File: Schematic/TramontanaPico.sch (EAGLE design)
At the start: 15 parts, among them U4 TEMT6000

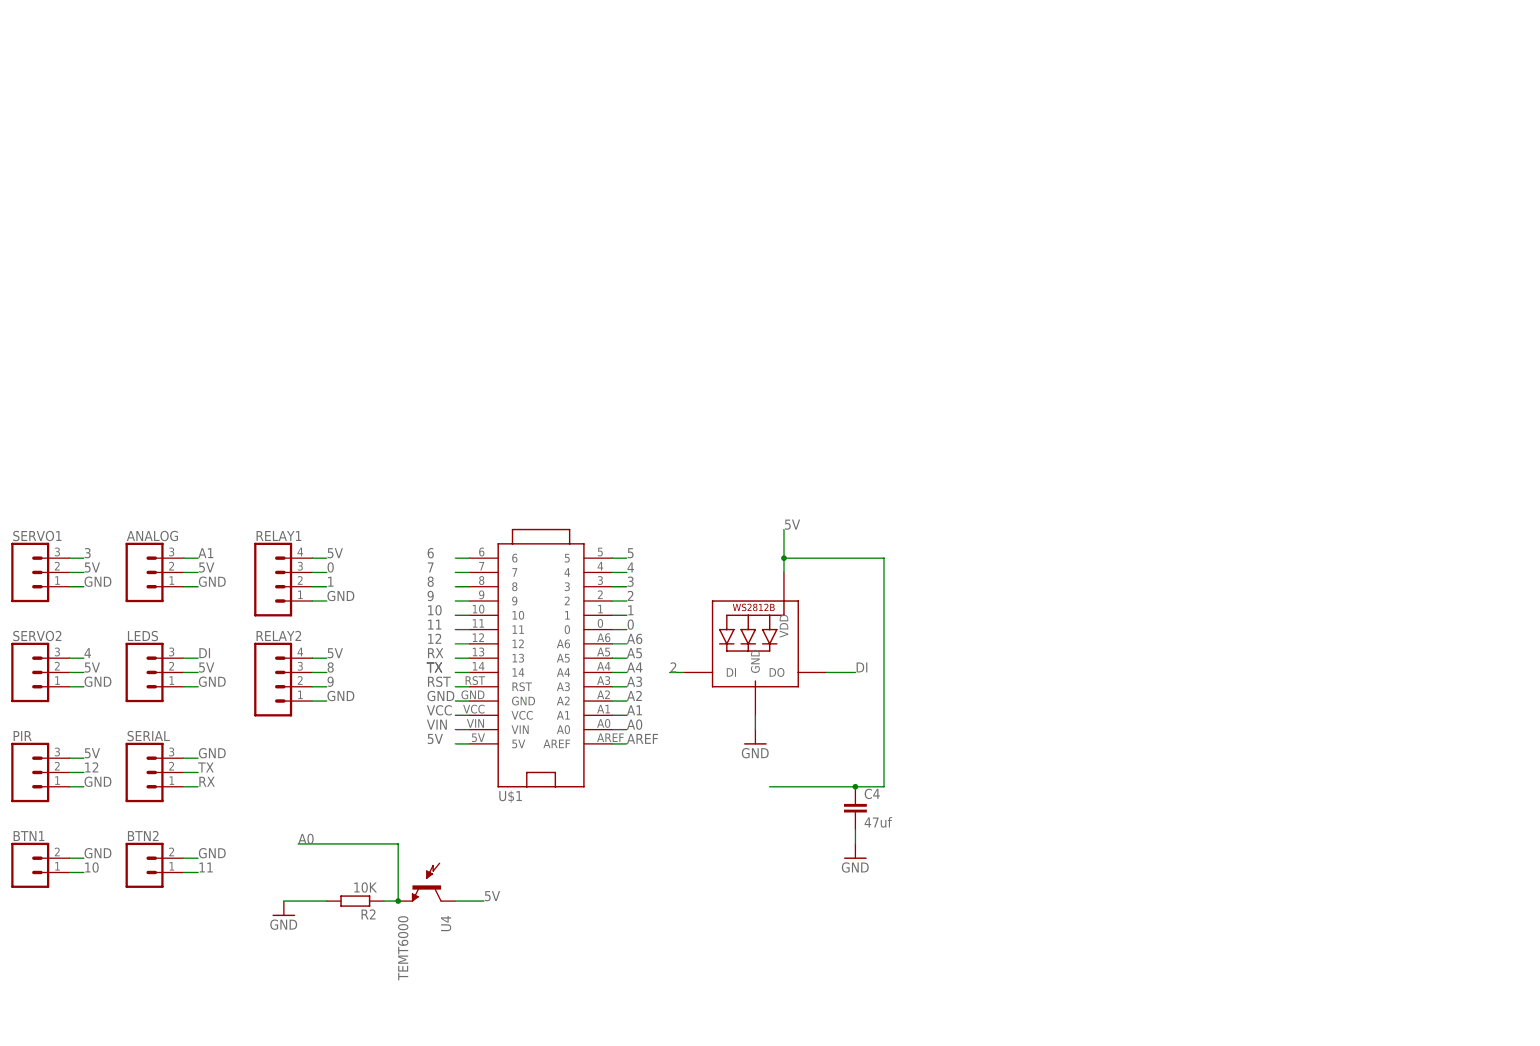
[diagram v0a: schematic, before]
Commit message: pier's version
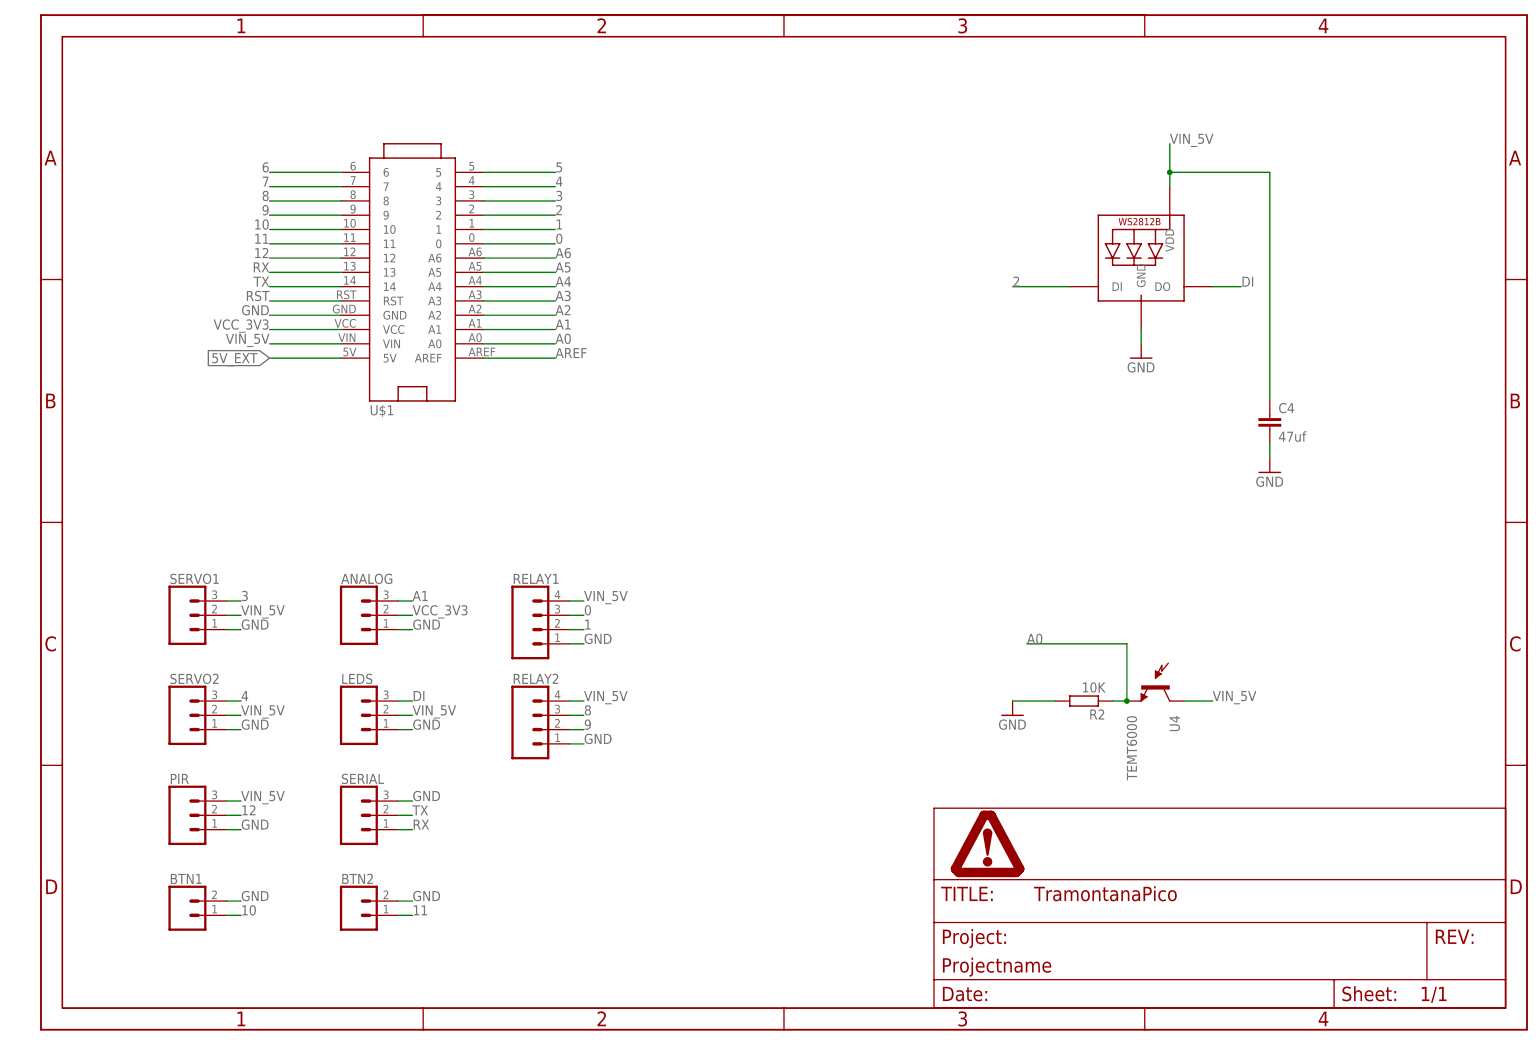
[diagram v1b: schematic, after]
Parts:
- added HTTP: FRAME_DINA4_L, dp_devices:FRAME_DINA4_L
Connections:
- removed net 5V: ANALOG.2, C4.1, LED1.VDD, LEDS.2, PIR.3, RELAY1.4, RELAY2.4, SERVO1.2, SERVO2.2, U$1.5V, U4.C1
- removed net VCC: U$1.VCC
- removed net VIN: U$1.VIN
- new net 5V_EXT: U$1.5V
- new net VCC_3V3: ANALOG.2, U$1.VCC
- new net VIN_5V: C4.1, LED1.VDD, LEDS.2, PIR.3, RELAY1.4, RELAY2.4, SERVO1.2, SERVO2.2, U$1.VIN, U4.C1
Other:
- moved on the sheet: ANALOG, BTN1, BTN2, C4, LEDS, PIR, R2, RELAY1, RELAY2, SERIAL, SERVO1, SERVO2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
